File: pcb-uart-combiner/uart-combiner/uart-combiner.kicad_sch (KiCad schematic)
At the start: 23 parts, among them J1 Conn_01x04, J2 Conn_01x04, J3 Conn_01x04, J4 Conn_01x04, J5 Conn_01x03, J6 Conn_01x03

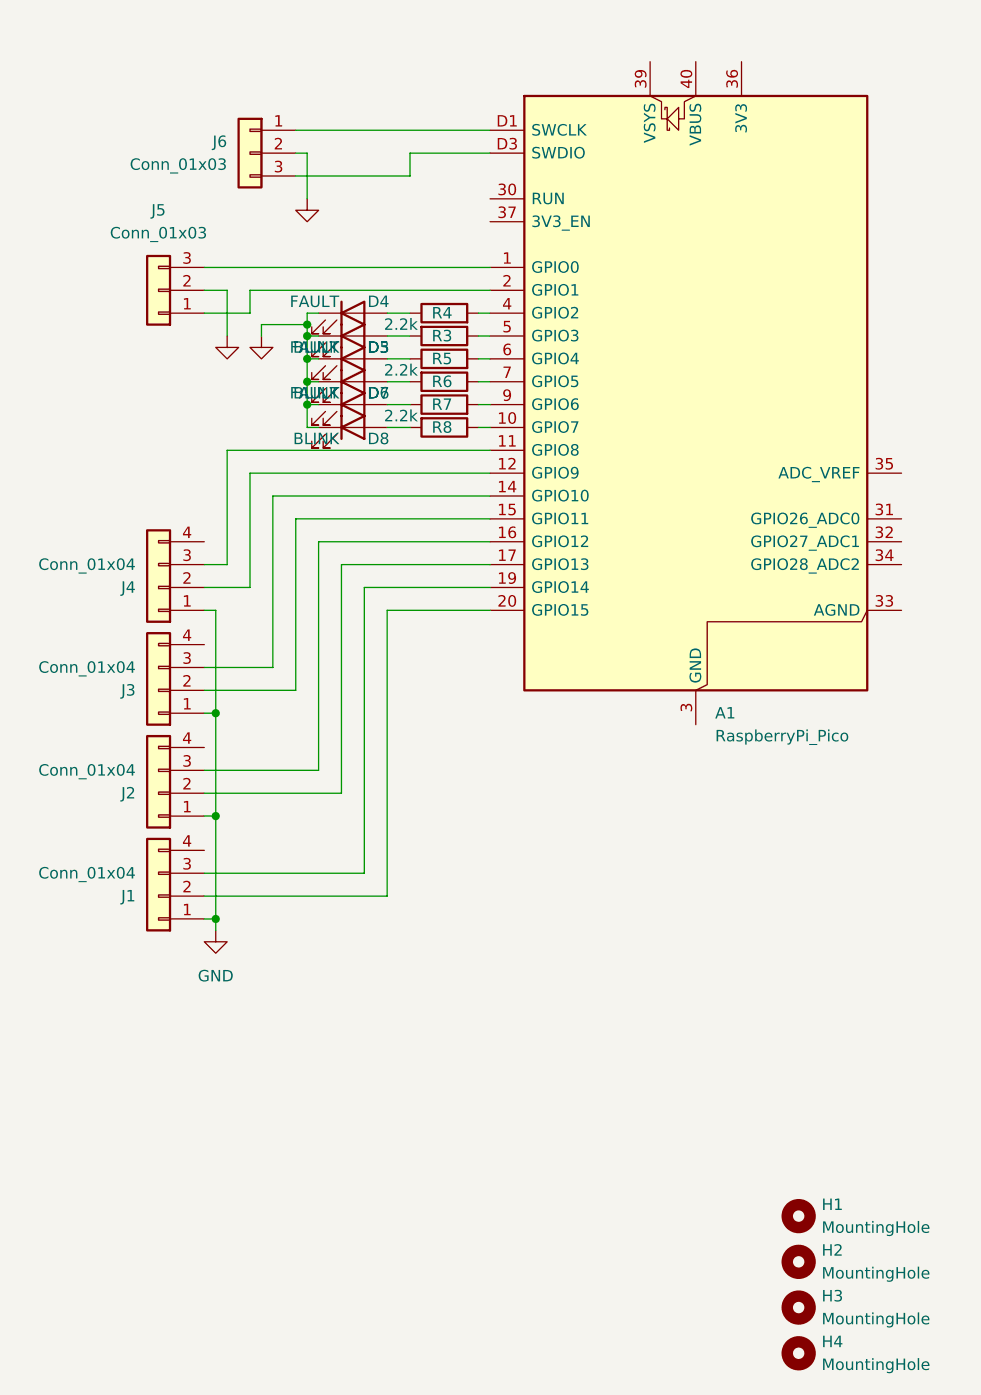
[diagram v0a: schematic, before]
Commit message: Working on MPPT combiner.
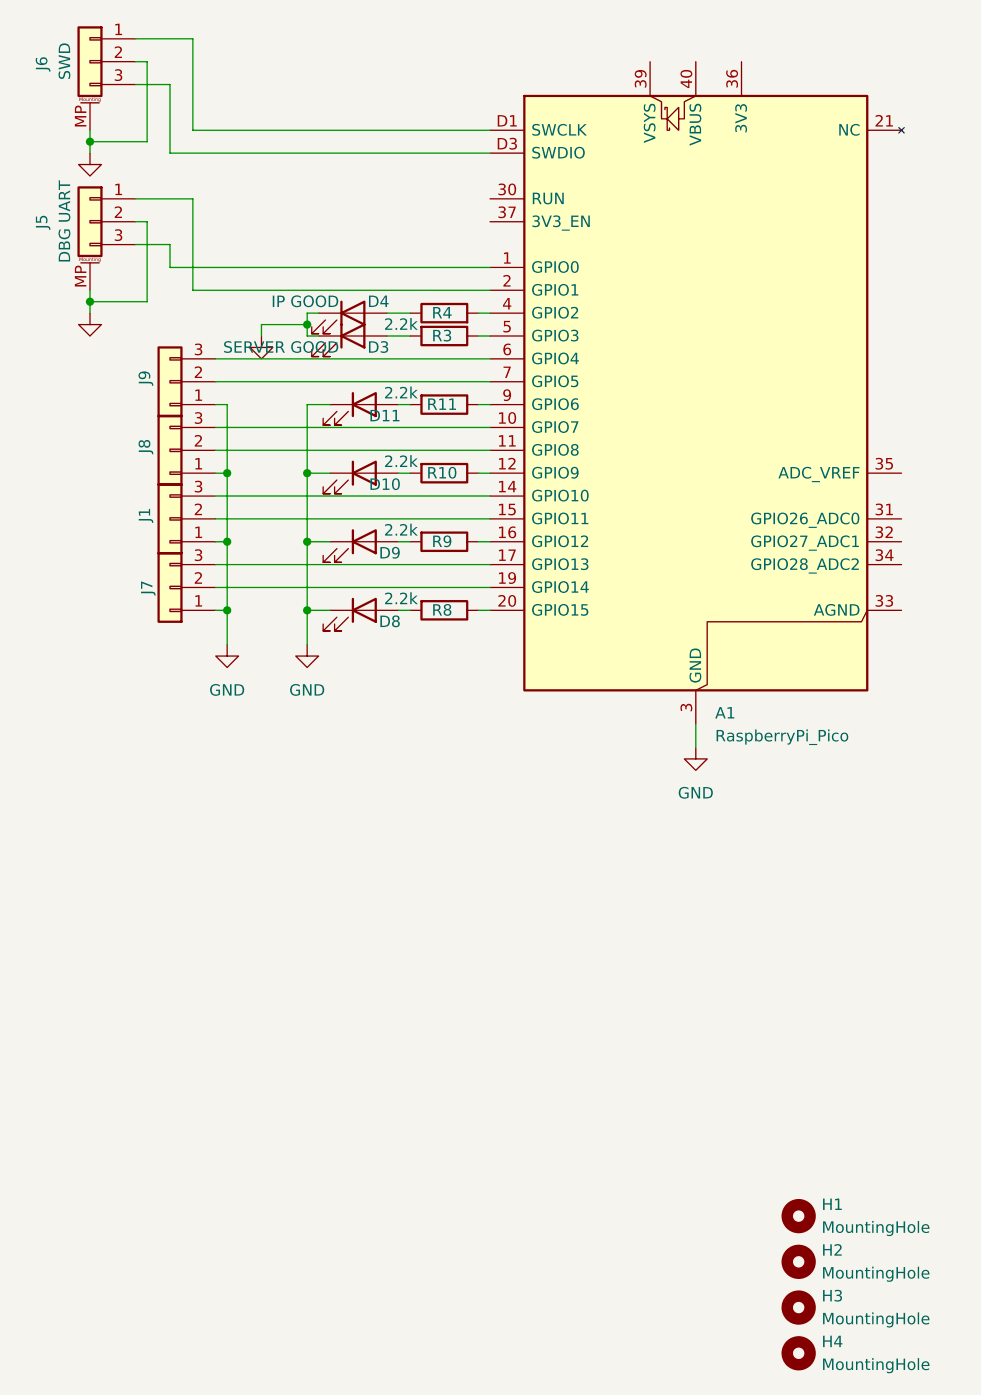
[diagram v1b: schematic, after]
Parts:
- removed D5, D7: FAULT, Diode_SMD:D_0603_1608Metric, symbol Device:LED
- removed D6: BLINK, Diode_SMD:D_0603_1608Metric, symbol Device:LED
- removed J1, J2, J3, J4: Conn_01x04, Connector_JST:JST_PH_B4B-PH-K_1x04_P2.00mm_Vertical, symbol Connector_Generic:Conn_01x04
- removed R5, R6, R7: 2.2k, Resistor_SMD:R_0603_1608Metric, symbol Device:R
- added D10, D11, D9: (no value), Diode_SMD:D_0603_1608Metric, symbol Device:LED
- added J1, J7, J8, J9: Conn_01x03, Connector_JST:JST_PH_B3B-PH-K_1x03_P2.00mm_Vertical, symbol Connector_Generic:Conn_01x03
- added R10, R11, R9: 2.2k, Resistor_SMD:R_0603_1608Metric, symbol Device:R
- D3: value BLINK -> SERVER GOOD
- D4: value FAULT -> IP GOOD
- D8: value BLINK -> (none)
- J5: value Conn_01x03 -> DBG UART; symbol Connector_Generic:Conn_01x03 -> Connector_Generic_MountingPin:Conn_01x03_MountingPin
- J6: value Conn_01x03 -> SWD; symbol Connector_Generic:Conn_01x03 -> Connector_Generic_MountingPin:Conn_01x03_MountingPin
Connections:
- net GND: now also A1.13 (GND), A1.18 (GND), A1.23 (GND), A1.28 (GND), A1.3 (GND), A1.38 (GND), A1.8 (GND), A1.D2 (GND), J5.MP (MountPin), J6.MP (MountPin), D10.1 (K), D11.1 (K), D9.1 (K), J1.1 (Pin_1), J7.1 (Pin_1), J8.1 (Pin_1), J9.1 (Pin_1)
- net at A1.15 (GPIO11): now also J1.2 (Pin_2)
- net at A1.14 (GPIO10): now also J1.3 (Pin_3)
- net at A1.12 (GPIO9): now also R10.1
- net at A1.11 (GPIO8): now also J8.2 (Pin_2)
- net at A1.7 (GPIO5): now also J9.2 (Pin_2)
- net at A1.17 (GPIO13): now also J7.3 (Pin_3)
- net at A1.16 (GPIO12): now also R9.1
- net at A1.9 (GPIO6): now also R11.1
- net at A1.10 (GPIO7): now also J8.3 (Pin_3); no longer R8.1
- net at A1.20 (GPIO15): now also R8.1
- net at A1.19 (GPIO14): now also J7.2 (Pin_2)
- net at A1.6 (GPIO4): now also J9.3 (Pin_3)
- new net: D9.2 (A), R9.2
- new net: D10.2 (A), R10.2
- new net: D11.2 (A), R11.2
- new net: A1.21 (NC), A1.22 (NC), A1.24 (NC), A1.25 (NC), A1.26 (NC), A1.27 (NC), A1.29 (NC)
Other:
- moved on the sheet: D8, R8
